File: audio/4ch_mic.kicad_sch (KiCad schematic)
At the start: 39 parts, among them J11 MIC1, J12 MIC2, J13 MIC3, J14 MIC4, U10 ac108, U11 TCR3RM33, U12 TCR3RM33, X1 ASE-24.000MHz

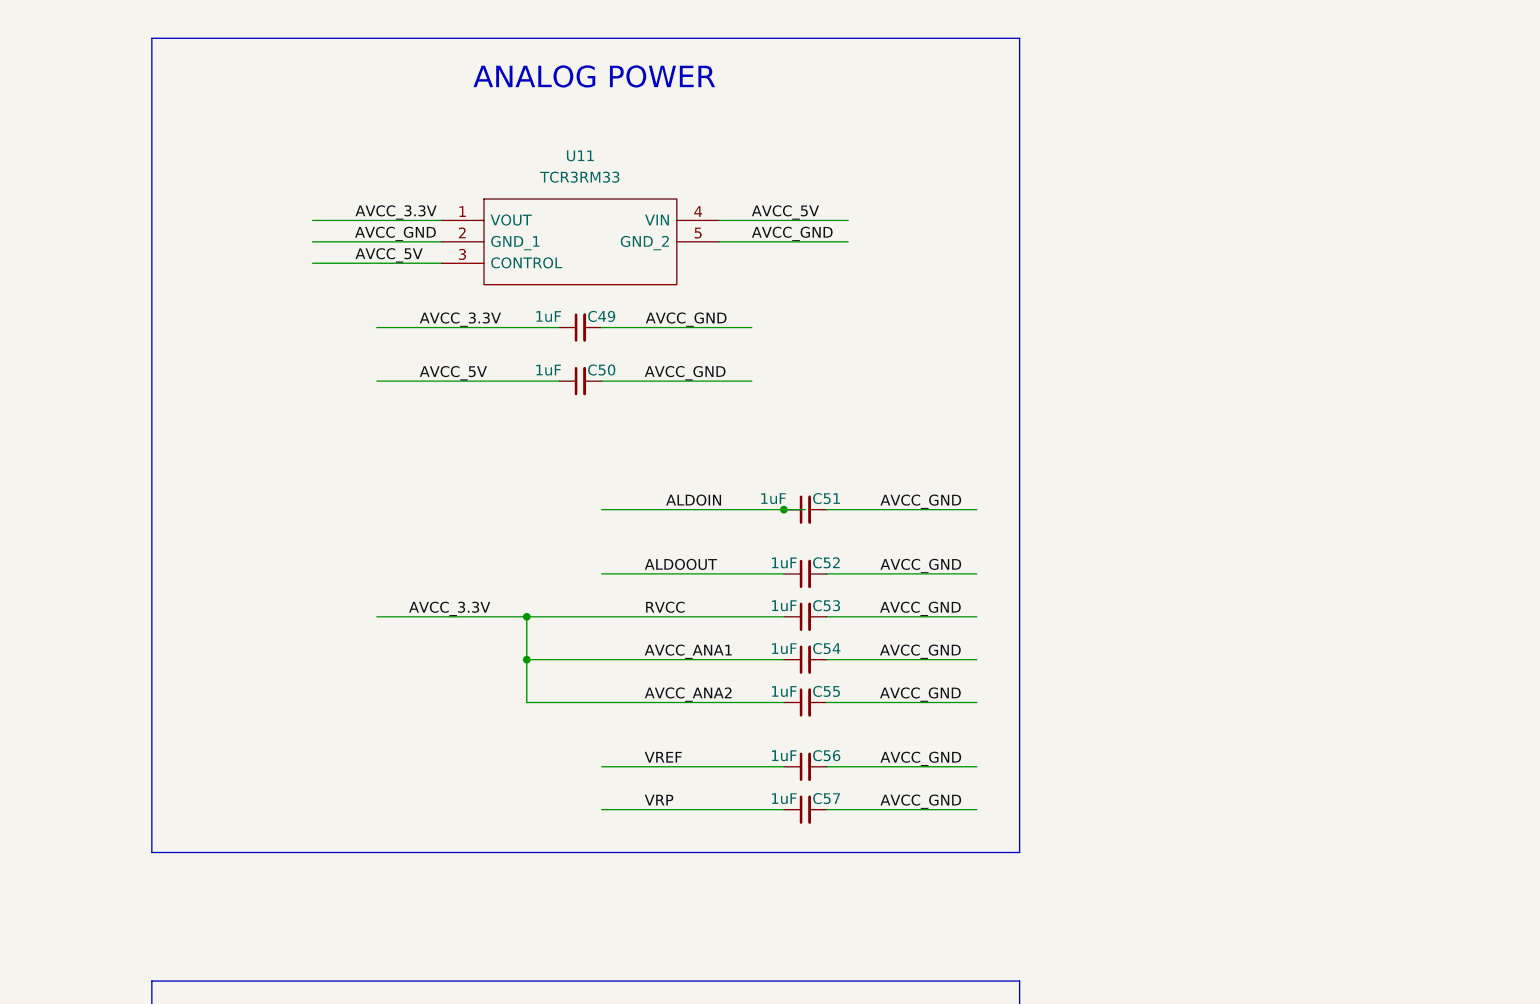
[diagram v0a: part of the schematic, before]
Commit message: .
.
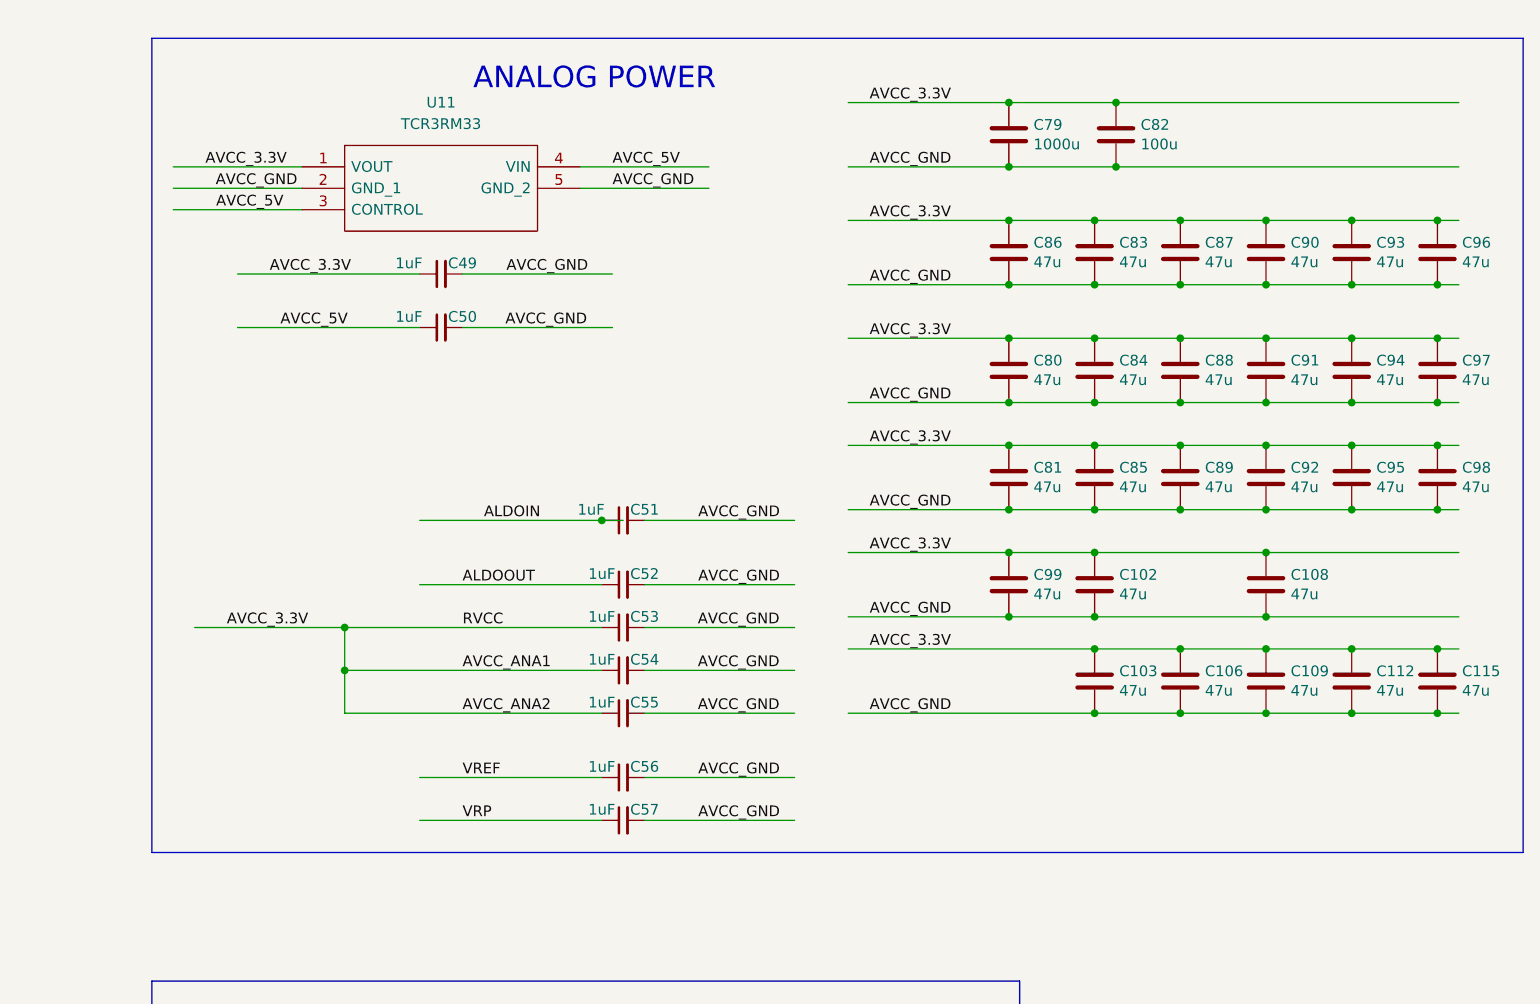
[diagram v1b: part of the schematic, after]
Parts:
- added C102, C103, C106, C108, C109, C112, C115, C80, C81, C83, C84, C85, C86, C87, C88, C89, C90, C91, C92, C93, C94, C95, C96, C97, C98, C99: 47u, Capacitor_SMD:C_0603_1608Metric, symbol Device:C
- added C79: 1000u, Capacitor_Tantalum_SMD:CP_EIA-7360-38_Kemet-E, symbol Device:C
- added C82: 100u, Capacitor_Tantalum_SMD:CP_EIA-3528-21_Kemet-B, symbol Device:C
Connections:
- net AVCC_3.3V: now also C102.1, C103.1, C106.1, C108.1, C109.1, C112.1, C115.1, C79.1, C80.1, C81.1, C82.1, C83.1, C84.1, C85.1, C86.1, C87.1, C88.1, C89.1, C90.1, C91.1, C92.1, C93.1, C94.1, C95.1, C96.1, C97.1, C98.1, C99.1
- net AVCC_GND: now also C102.2, C103.2, C106.2, C108.2, C109.2, C112.2, C115.2, C79.2, C80.2, C81.2, C82.2, C83.2, C84.2, C85.2, C86.2, C87.2, C88.2, C89.2, C90.2, C91.2, C92.2, C93.2, C94.2, C95.2, C96.2, C97.2, C98.2, C99.2
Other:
- moved on the sheet: C49, C50, C51, C52, C53, C54, C55, C56, C57, U11
